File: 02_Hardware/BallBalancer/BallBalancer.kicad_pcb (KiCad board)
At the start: 2 copper layers, 64.5 x 77 mm, 128 parts, among them J1 USB_B_Micro, J2 Raspberry PI UART, J3 SWD, J4 Reference switch 1, J5 ENCODER 1, J6 ENCODER 2, J7 Reference switch 2, J8 Jack-DC, M1 Motor_DC, M2 Motor_DC, Q1 DMN10H220L, Q2 DMN10H220L, Q3 DMN10H220L, Q4 DMN10H220L, Q5 DMN10H220L, Q6 DMN10H220L, Q7 DMN10H220L, Q8 DMN10H220L, U1 STM32L412K8Tx, U2 USBLC6-2SC6, U3 DGD0506A, U4 DGD0506A, U5 LM2937IMP5, U6 AP63203WU, U7 DGD0506A, U8 DGD0506A

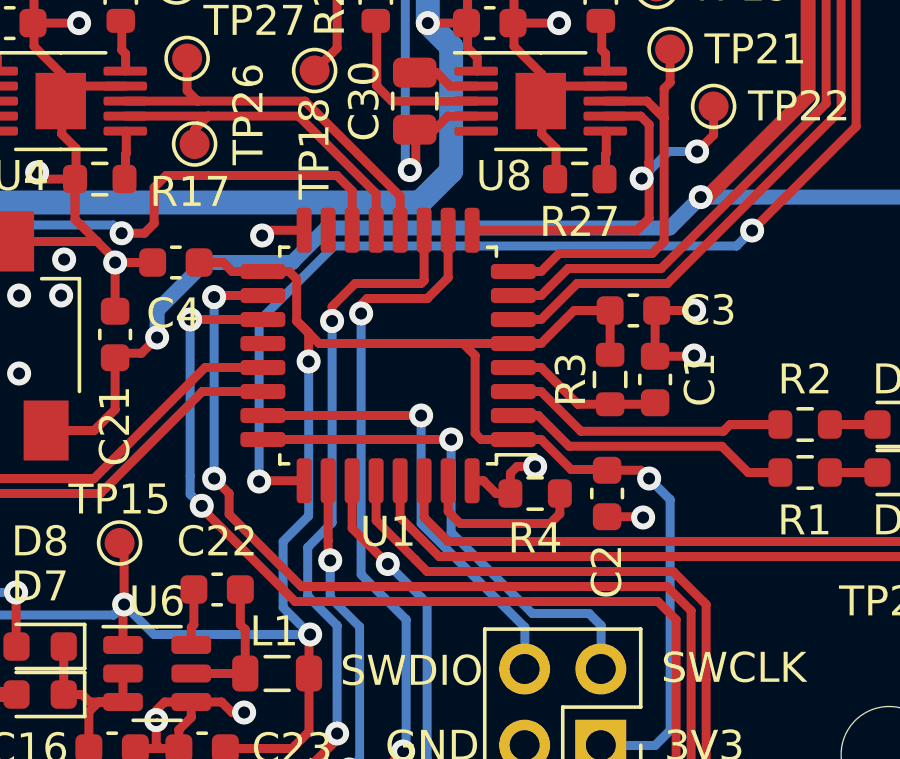
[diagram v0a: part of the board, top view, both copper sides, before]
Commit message: CAD files and hardware manufacturing data added
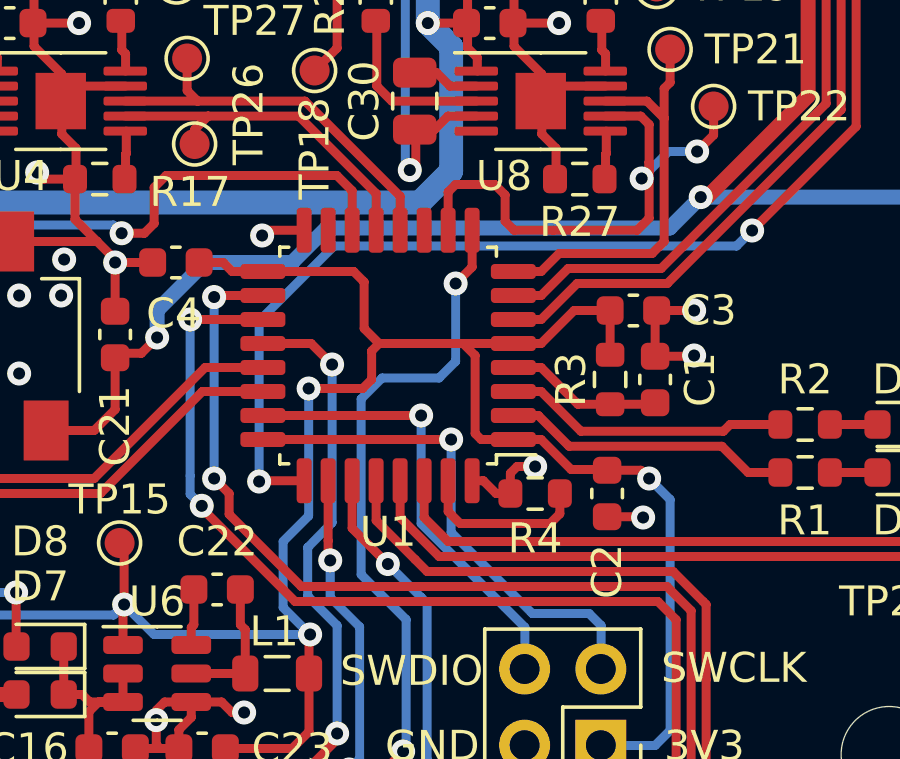
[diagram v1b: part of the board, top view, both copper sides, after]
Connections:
- U1 pad 10: IN_MOT_CH1L -> EN_MOT_CH2R
- U1 pad 11: IN_MOT_CH1R -> unconnected-(U1-PA5-Pad11)
- U1 pad 20: unconnected-(U1-PA10-Pad20) -> IN_MOT_CH1R
- U1 pad 9: EN_MOT_CH2R -> IN_MOT_CH1L
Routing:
- net IN_MOT_CH1R: track 48.1 -> 43.7 mm
- net EN_MOT_CH2R: track 15.4 -> 18.7 mm
- net +3V3: track 92.5 -> 93.7 mm
